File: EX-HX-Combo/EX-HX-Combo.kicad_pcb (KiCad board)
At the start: 2 copper layers, 150.2 x 124.5 mm, 45 parts, among them CN1 DB9 Male, J1 IDE_CONNECTOR, J200 Bus_Tandy_Plus_Through, J3 Bus_Tandy_Plus, SW1 SW_DIP_x10, U1 BIOS FLASH, U2 74HCT245, U3 1.8432 MHz, U4 DS1315, U5 AS6C4008-55PCN, U6 16550/16C550, U7 GD75232N, U8 GAL16V8, U9 GAL16V8, Y1 32.768 KHz

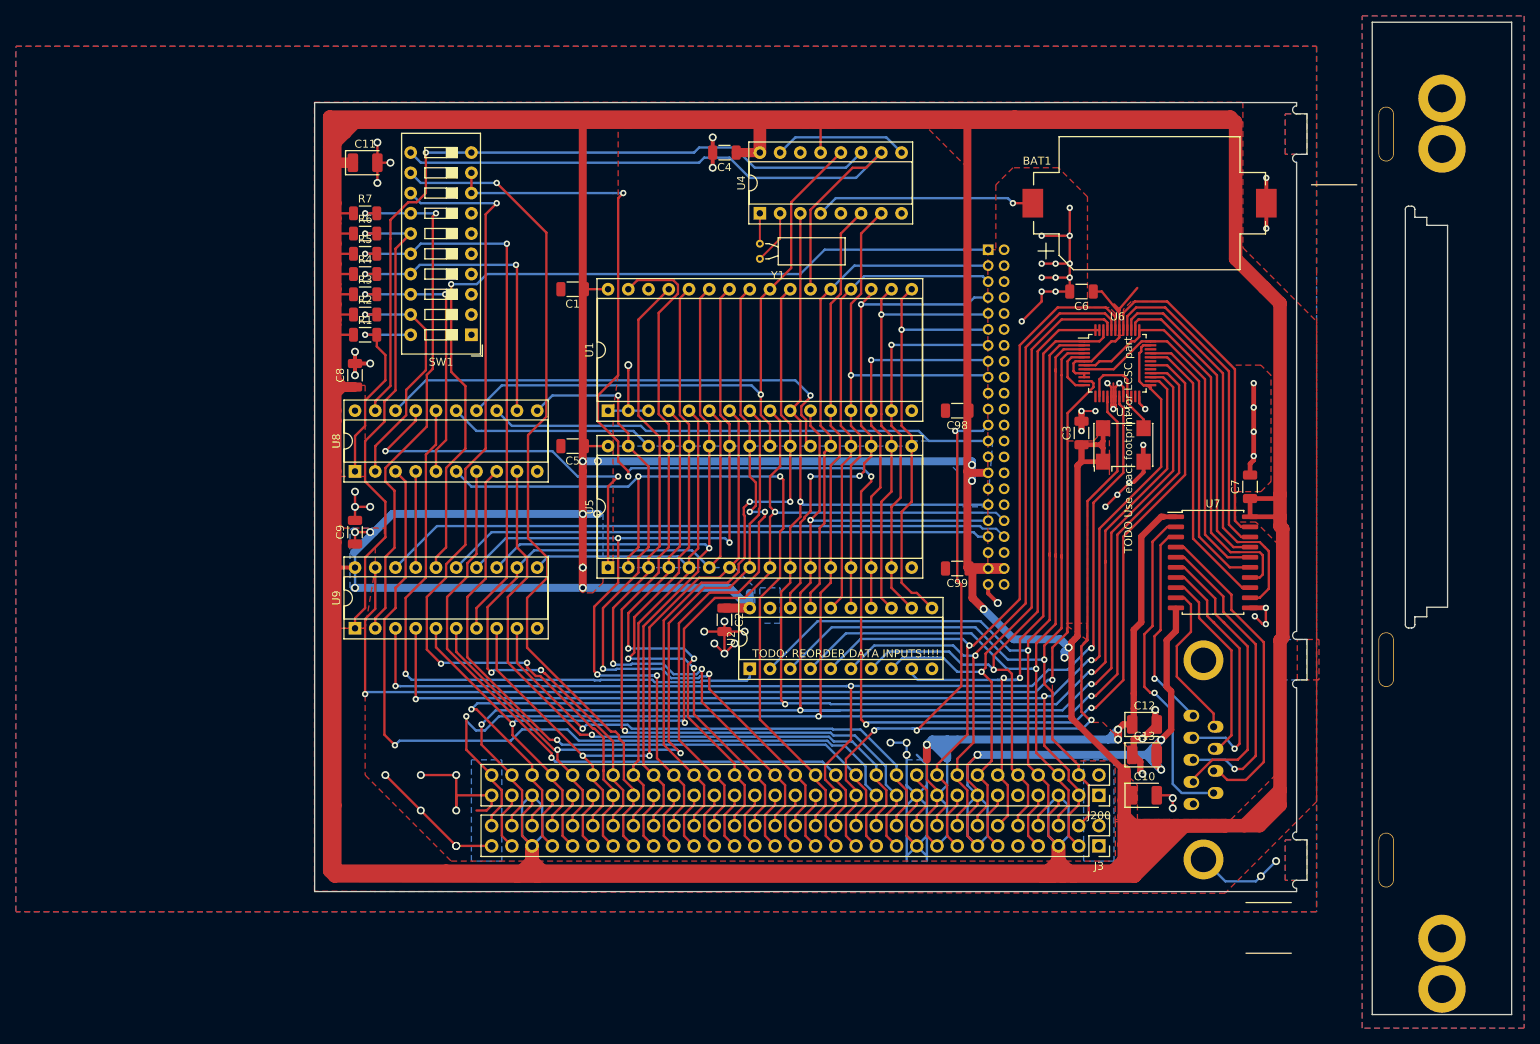
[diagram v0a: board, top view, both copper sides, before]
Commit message: More EX-HX Combo layout work.
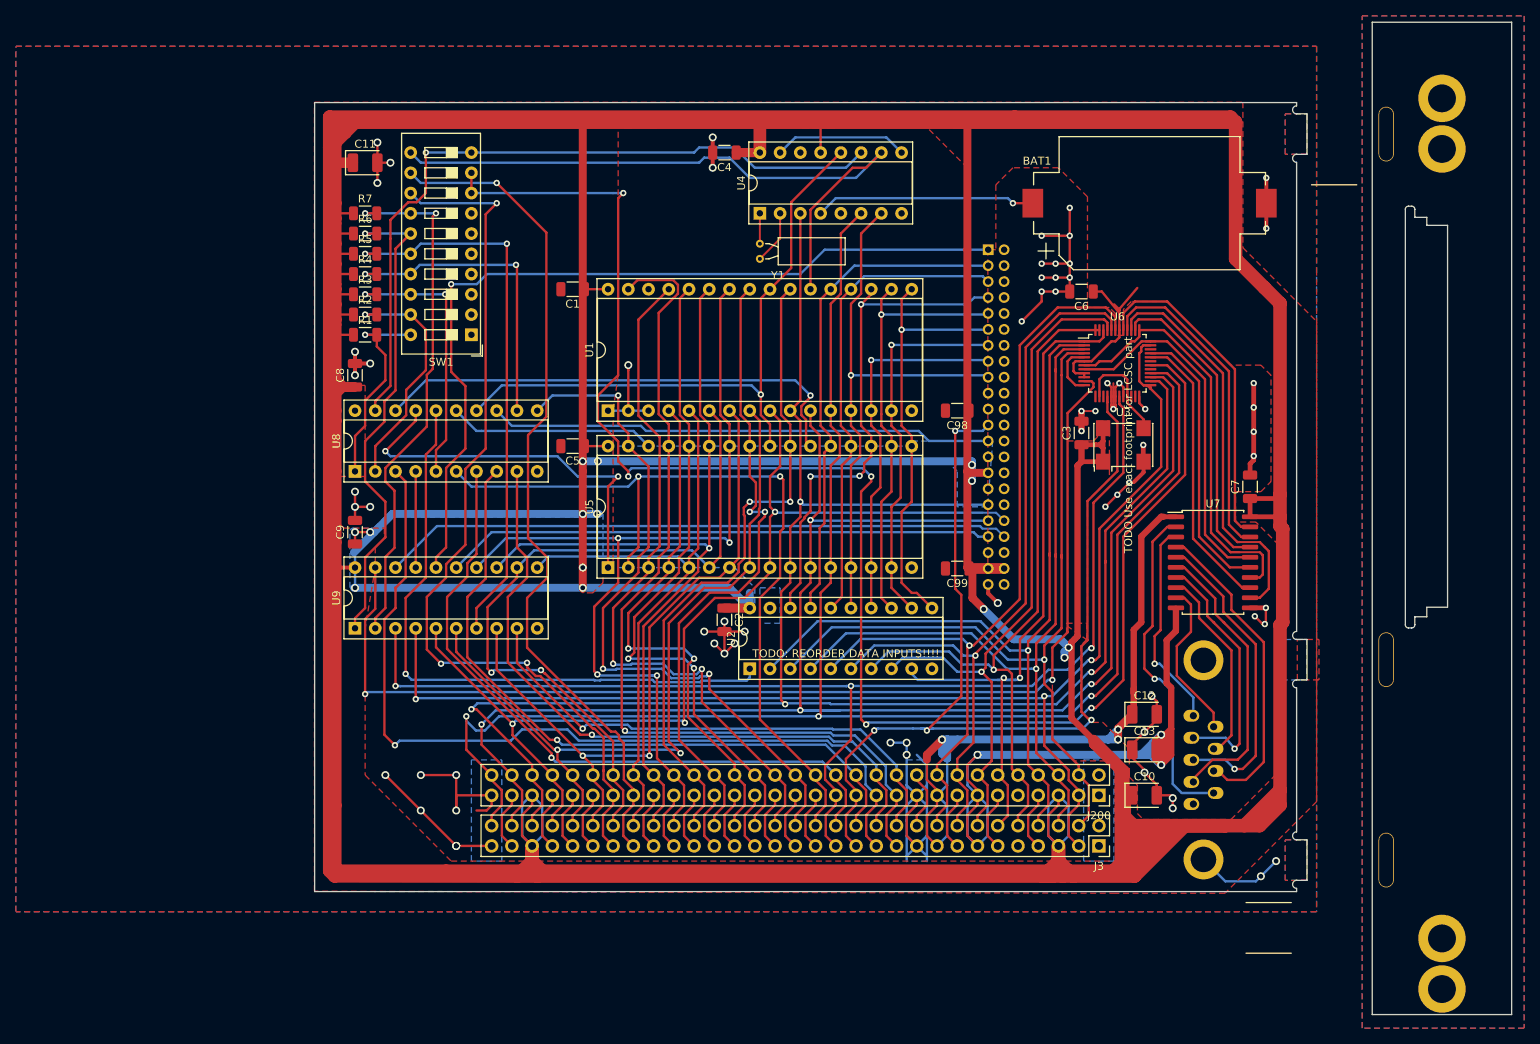
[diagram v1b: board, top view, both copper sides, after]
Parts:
- moved C12 1.27 mm to (224.2, 114.3)
- moved C13 0.63 mm to (224.2, 118.7)
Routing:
- net VCC: track 1288.1 -> 1307.0 mm
- net -12V: track 84.5 -> 100.4 mm
- net +12V: track 102.8 -> 96.7 mm
- net GND: track 245.8 -> 250.9 mm
